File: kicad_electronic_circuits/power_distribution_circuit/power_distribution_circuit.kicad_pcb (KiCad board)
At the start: 2 copper layers, 8 parts, among them J2 Conn_01x04, J3 Conn_01x02, J4 Conn_01x02, J5 Conn_01x04, J6 Conn_01x04, J7 Conn_01x02, J8 Conn_01x02, J9 Conn_01x04

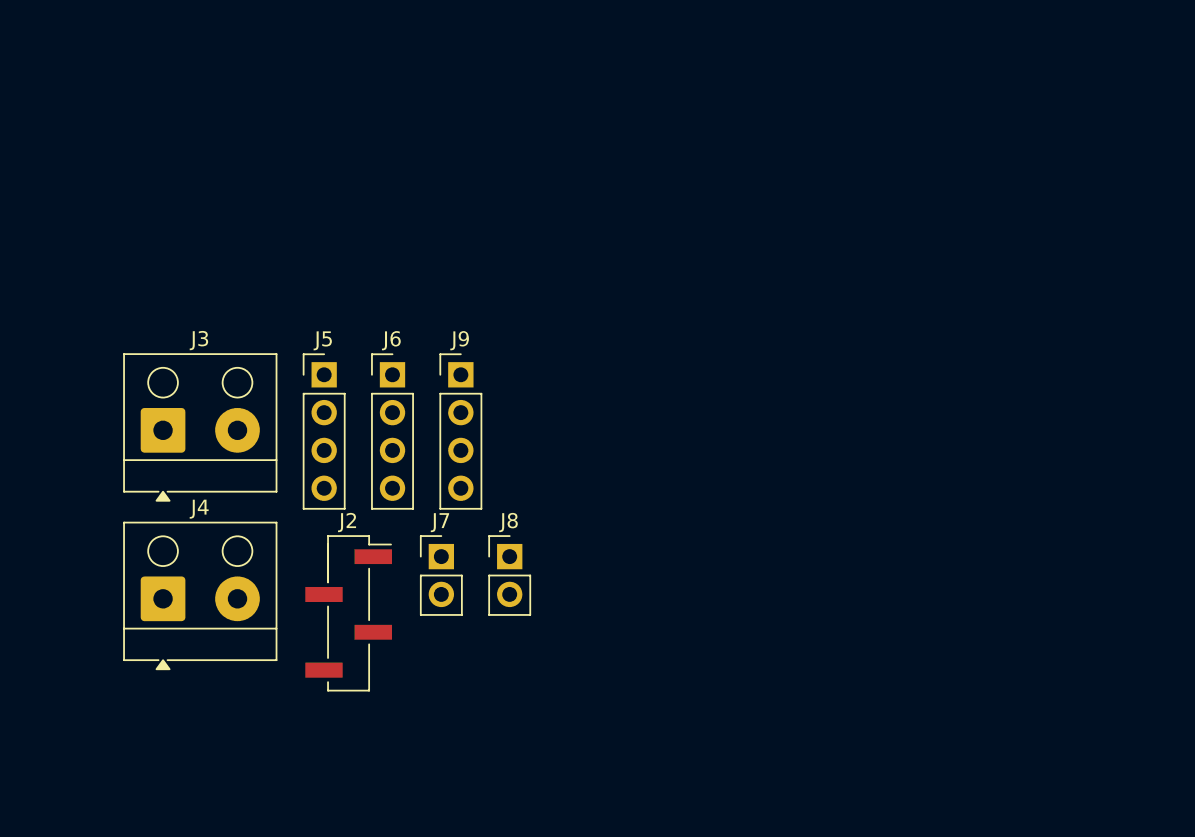
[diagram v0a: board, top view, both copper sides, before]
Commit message: qu
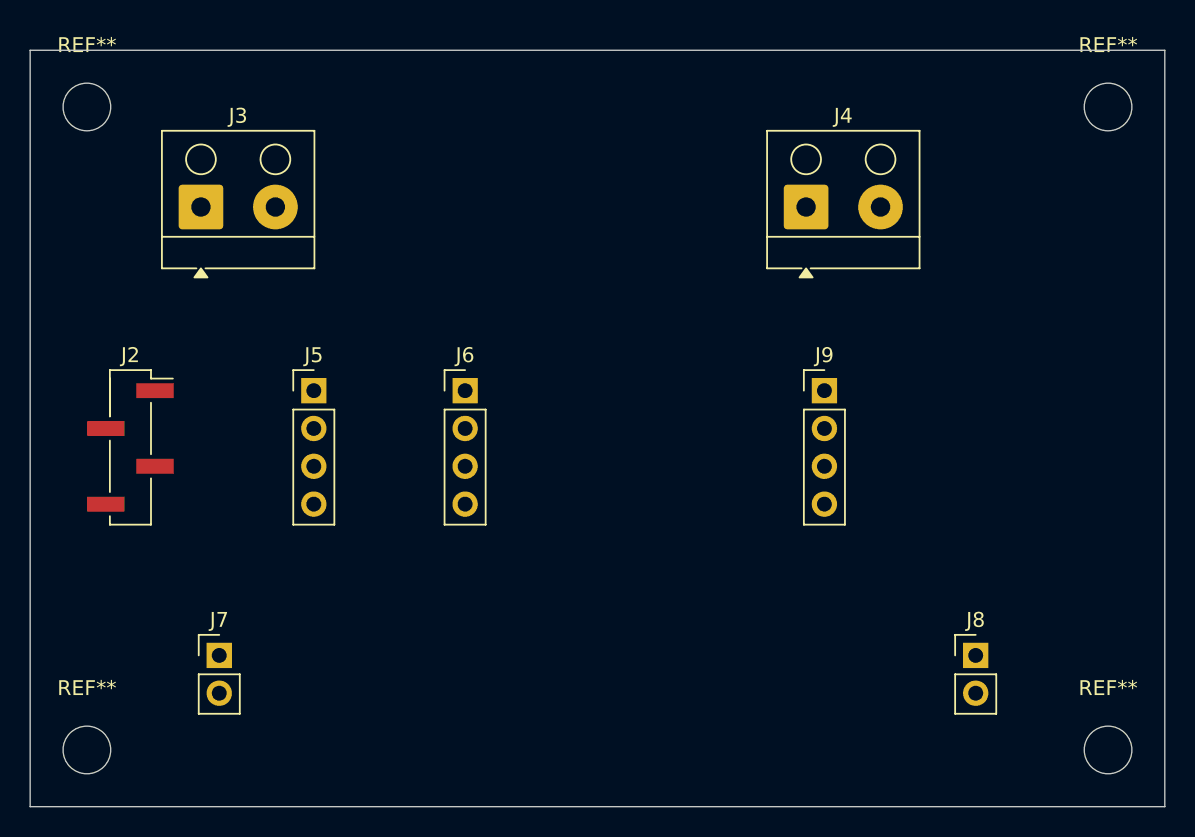
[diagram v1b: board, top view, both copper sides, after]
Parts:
- added REF**: MountingHole_3.2mm_M3, MountingHole:MountingHole_3.2mm_M3, F.Cu at (105.4, 67.3)
- added REF**: MountingHole_3.2mm_M3, MountingHole:MountingHole_3.2mm_M3, F.Cu at (105.4, 110.5)
- added REF**: MountingHole_3.2mm_M3, MountingHole:MountingHole_3.2mm_M3, F.Cu at (174.0, 67.3)
- added REF**: MountingHole_3.2mm_M3, MountingHole:MountingHole_3.2mm_M3, F.Cu at (174.0, 110.5)
- moved J4 50.6 mm to (153.7, 74.0)
- moved J8 32.0 mm to (165.1, 104.1)
- moved J9 24.4 mm to (154.9, 86.4)
- moved J2 18.4 mm to (108.3, 90.2)
- moved J7 16.3 mm to (114.3, 104.1)
- moved J3 15.2 mm to (113.1, 74.0)
- moved J6 4.99 mm to (130.8, 86.4)
- moved J5 1.27 mm to (120.7, 86.4)
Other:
- board outline added: 76.2 x 50.8 mm
